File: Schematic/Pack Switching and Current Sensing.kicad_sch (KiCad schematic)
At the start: 31 parts, among them Q10 CSD19531Q5A, Q11 ZXMP10A13F, Q12 CSD19531Q5A, Q13 CSD19531Q5A, Q9 CSD19531Q5A

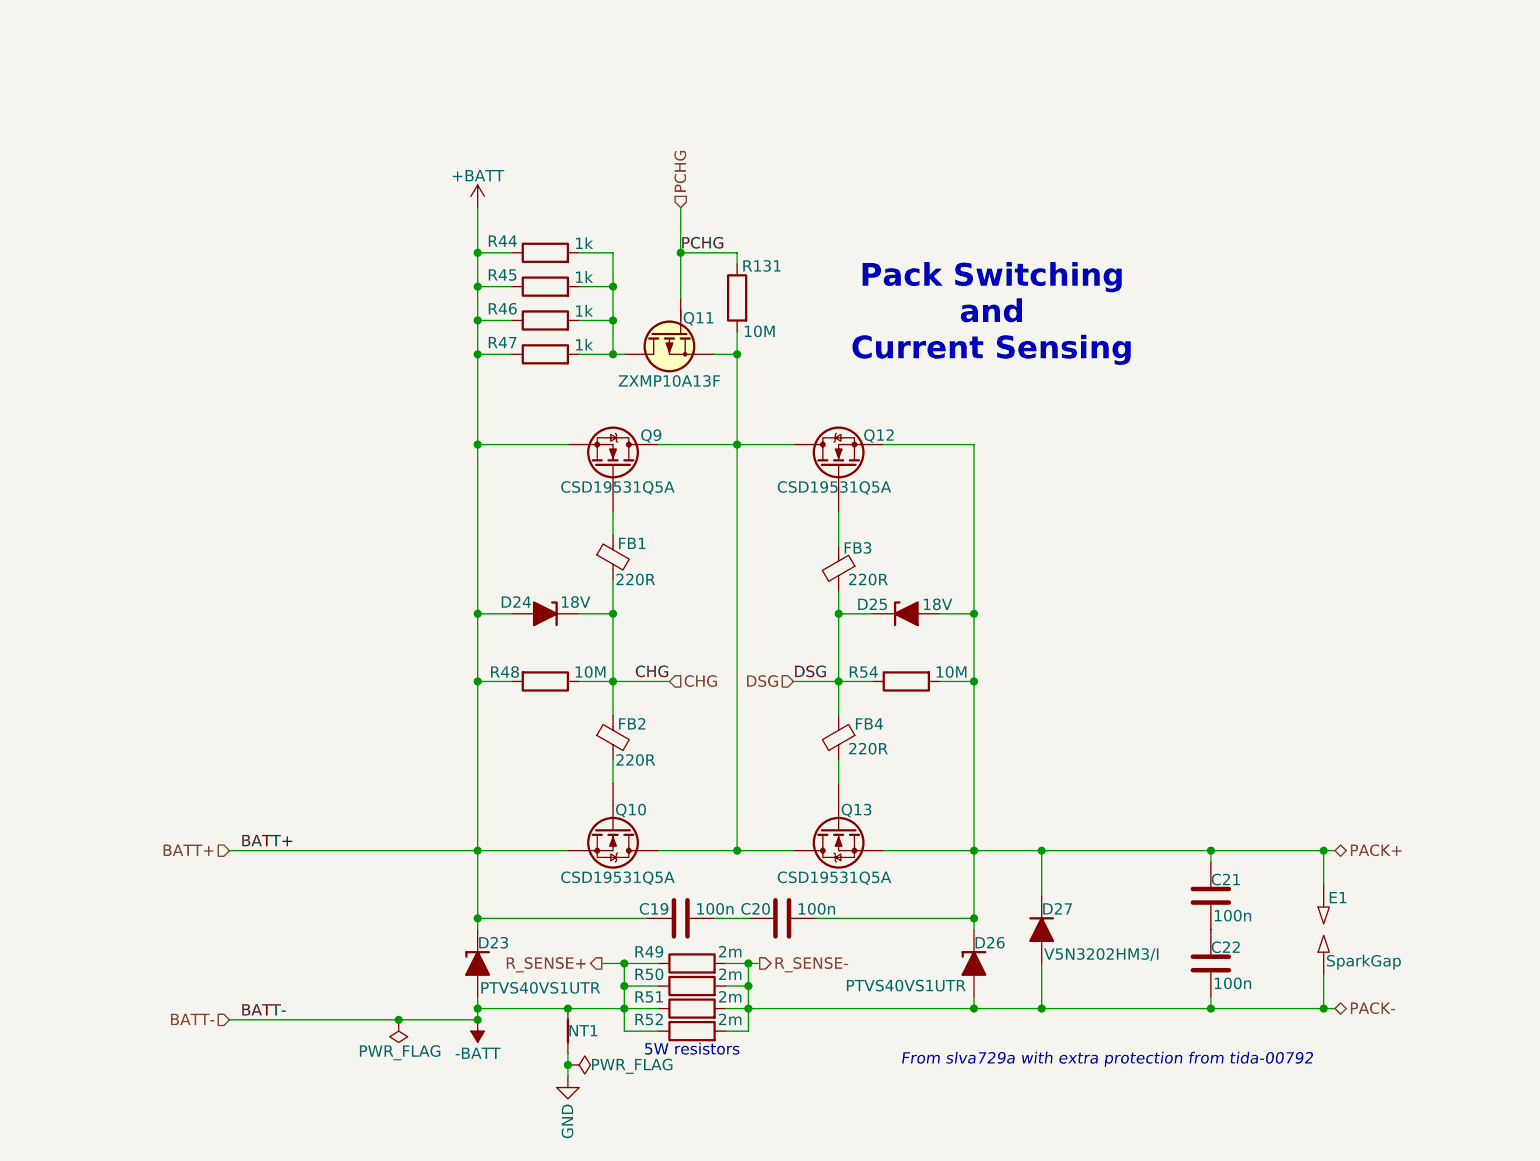
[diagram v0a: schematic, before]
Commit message: added sensors?
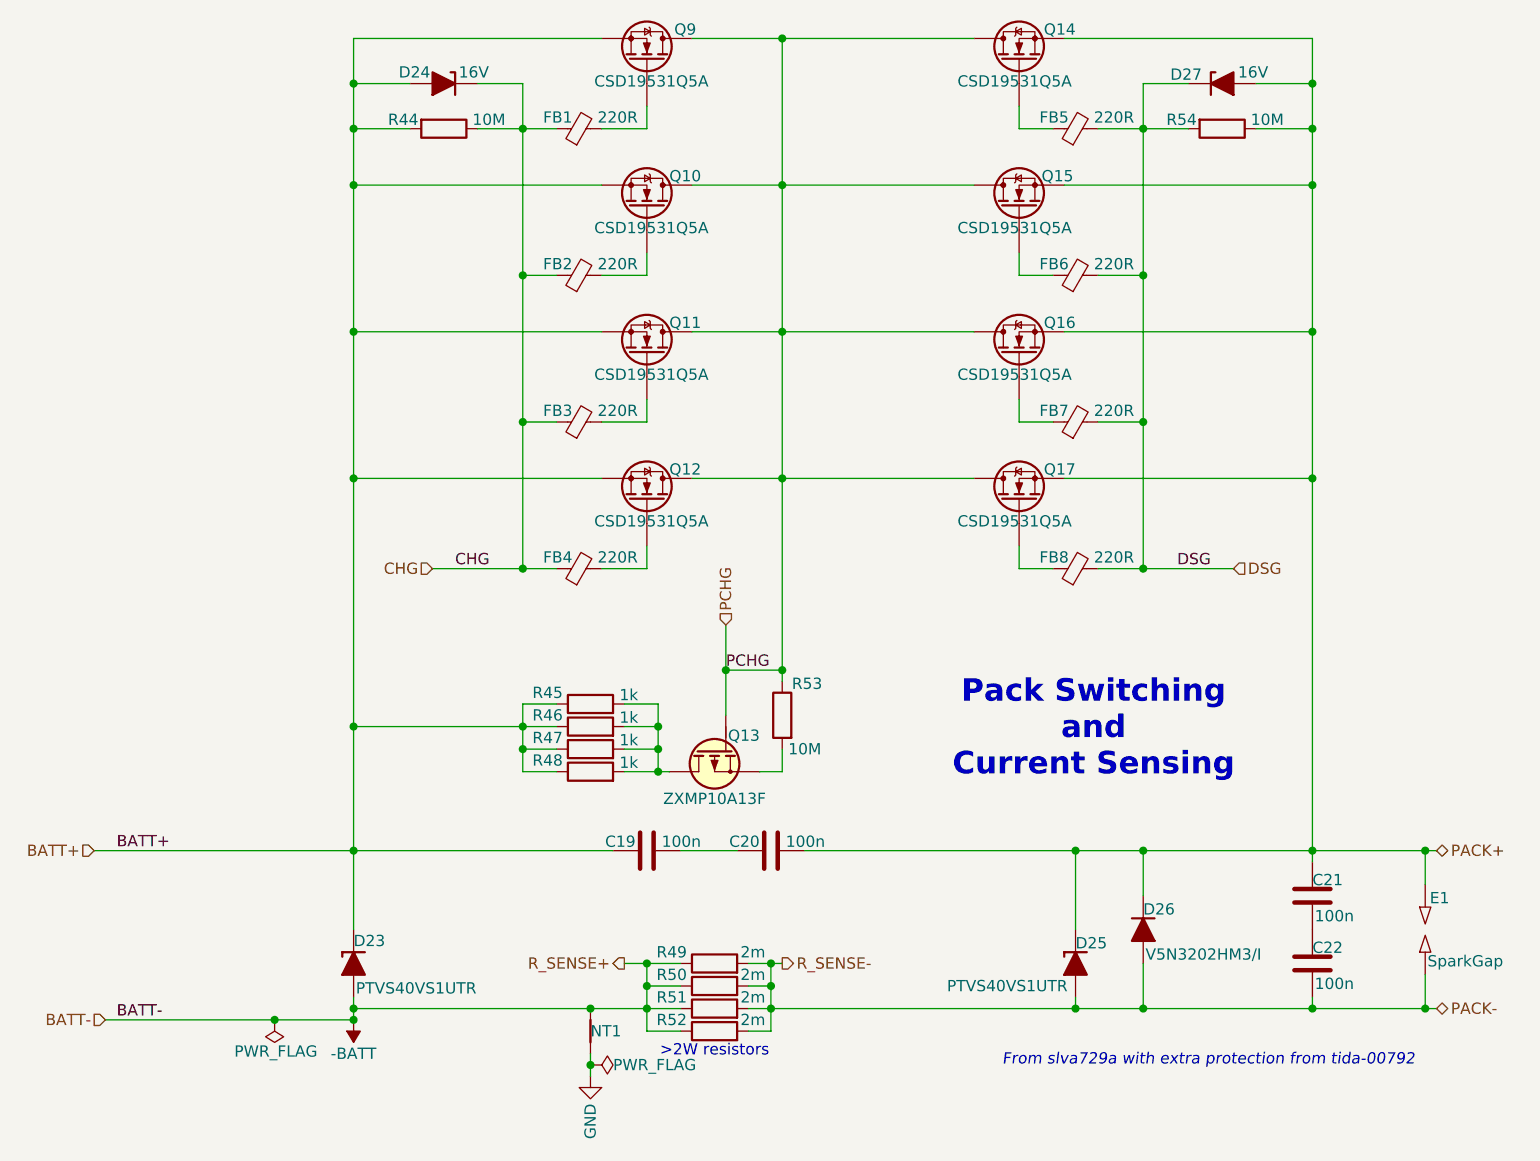
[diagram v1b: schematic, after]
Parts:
- removed D25: 18V, symbol Device:D_Zener_Filled
- removed Q13: CSD19531Q5A, Package_TO_SOT_SMD:TDSON-8-1, symbol Transistor_FET:CSD19531Q5A
- removed R44: 1k, symbol Device:R
- added D27: 16V, symbol Device:D_Zener_Filled
- added FB5, FB6, FB7, FB8: 220R, symbol Device:FerriteBead_Small
- added Q11, Q14, Q15, Q16, Q17: CSD19531Q5A, Package_TO_SOT_SMD:TDSON-8-1, symbol Transistor_FET:CSD19531Q5A
- added R47: 1k, symbol Device:R
- D24: value 18V -> 16V
- renumbered D26 to D25, D27 to D26, Q11 to Q13, R48 to R44, R47 to R48, R131 to R53
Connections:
- net CHG: now also FB1.1, FB3.1, FB4.1; no longer FB1.2
- net DSG: now also R54.2, D27.1 (K), FB5.2, FB6.2, FB7.2, FB8.2; no longer FB3.2, FB4.1, R54.1
- net PACK+: now also R54.1, D27.2 (A), Q14.1 (S), Q14.2 (S), Q14.3 (S), Q15.1 (S), Q15.2 (S), Q15.3 (S), Q16.1 (S), Q16.2 (S), Q16.3 (S), Q17.1 (S), Q17.2 (S), Q17.3 (S); no longer Q12.1 (S), Q12.2 (S), Q12.3 (S), R54.2
- net PCHG: now also Q10.5 (D), Q12.5 (D), Q9.5 (D), Q11.5 (D), Q14.5 (D), Q15.5 (D), Q16.5 (D), Q17.5 (D)
- net at FB4.2: now also Q12.4 (G)
- net at Q13.3 (D), R45.2, R46.2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: now also R47.2
- net at Q9.4 (G): now also FB1.2; no longer FB1.1
- net +BATT renamed BATT+
- net BATT+: now also Q12.1 (S), Q12.2 (S), Q12.3 (S), Q11.1 (S), Q11.2 (S), Q11.3 (S), R47.1
- new net: Q13.2 (S), R53.2
- new net: FB6.1, Q15.4 (G)
- new net: FB5.1, Q14.4 (G)
- new net: FB7.1, Q16.4 (G)
- new net: FB8.1, Q17.4 (G)
- new net: FB3.2, Q11.4 (G)
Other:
- note added: ">2W resistors"
- note removed: "5W resistors"
- moved on the sheet: C19, C20, C21, C22, D23, D24, D25, D26, E1, FB1, NT1, Q13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
